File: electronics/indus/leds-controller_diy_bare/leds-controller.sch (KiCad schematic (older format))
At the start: 18 parts, among them P1 ALIM_12V_60V, P10 THERM_LEDS, P2 MICRO_CTRL, P3 FANS, P4 POT_COLOR2, P5 POT_COLOR3, P6 POT_COLOR4, P7 POT_COLOR1, P8 LED+, P9 LED-

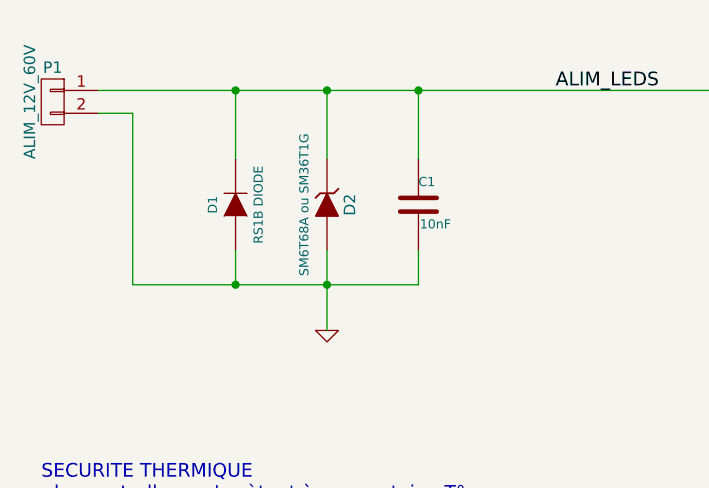
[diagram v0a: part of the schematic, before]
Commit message: bom refs etc
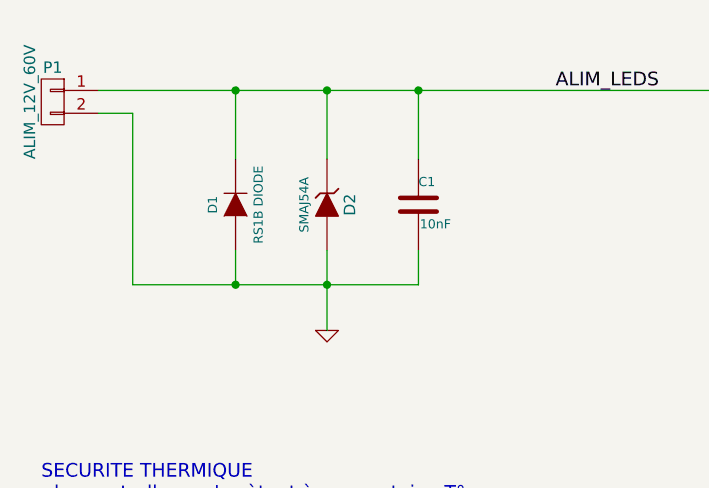
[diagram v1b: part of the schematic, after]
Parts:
- D2: value SM6T68A ou SM36T1G -> SMAJ54A
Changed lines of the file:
@@
 P 2050 1350
 F 0 "D2" H 2050 1450 50  0000 C CNN
-F 1 "SM6T68A ou SM36T1G" H 2050 1250 40  0000 C CNN
+F 1 "SMAJ54A" H 2050 1250 40  0000 C CNN
 F 2 "risebox:DIODE_DO_214_AA" H 2050 1350 60  0001 C CNN
 F 3 "" H 2050 1350 60  0000 C CNN
